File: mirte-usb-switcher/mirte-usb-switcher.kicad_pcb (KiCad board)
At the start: 2 copper layers, 18.4 x 27.4 mm, 5 parts, among them J1 Conn_02x02_Counter_Clockwise, U1 SIP32509DT-T1-GE3

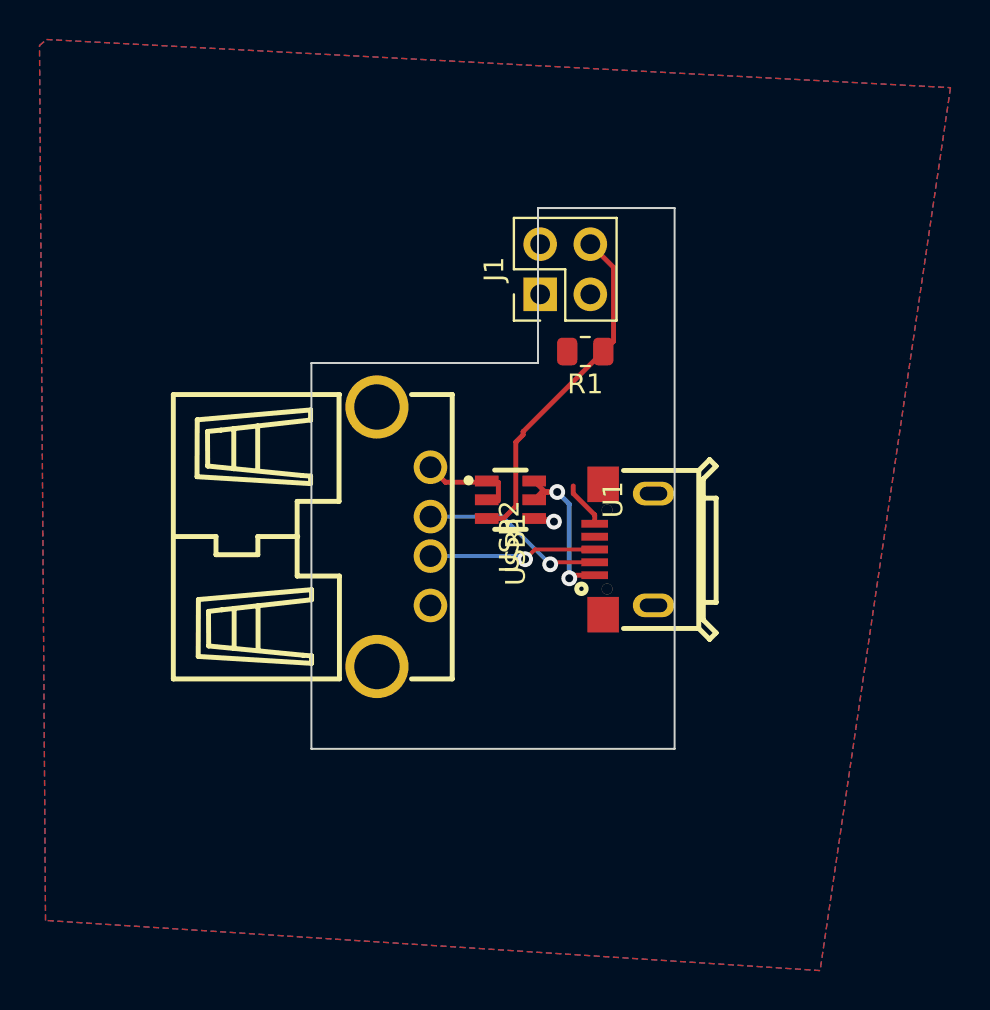
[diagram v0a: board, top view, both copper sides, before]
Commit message: move usb switcher
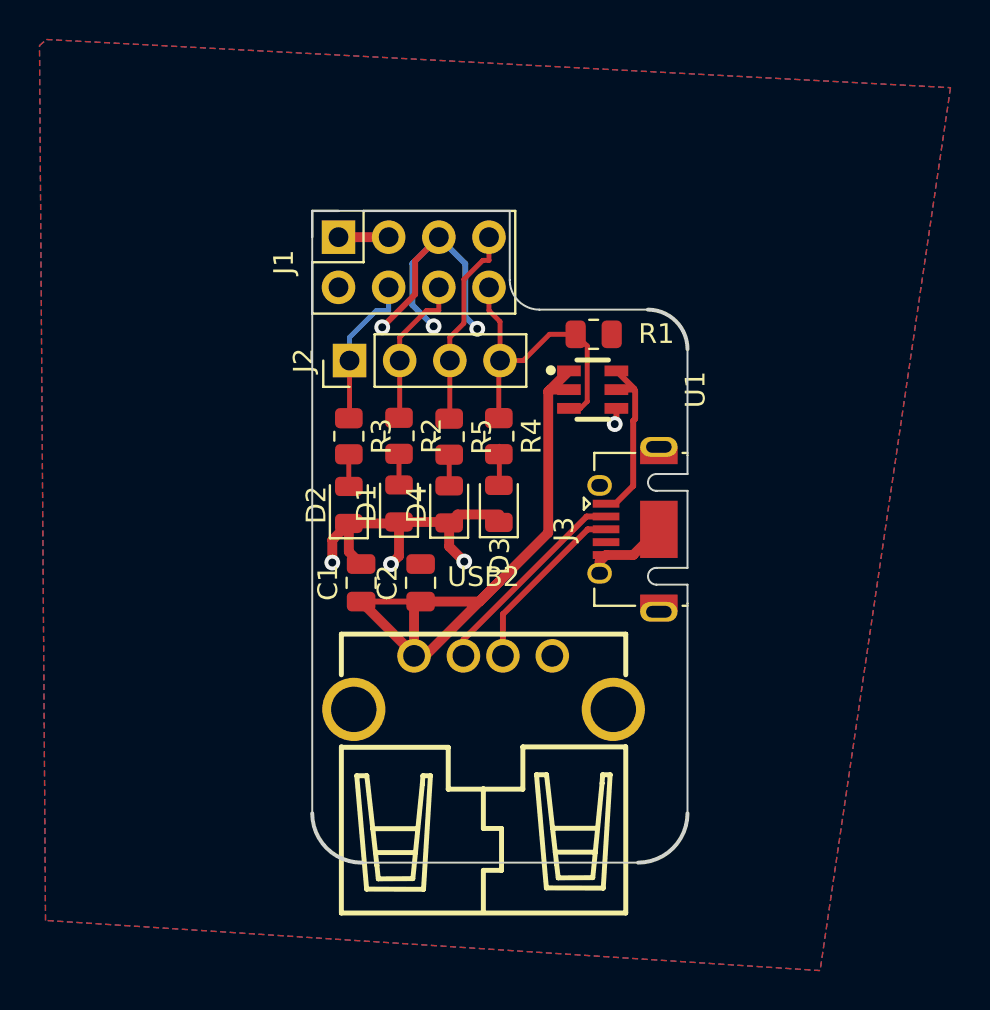
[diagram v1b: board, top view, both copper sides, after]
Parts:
- removed USB1: U254-051T-4BH83-S1S, lcsc:MICRO-USB-SMD_U254-051T-4BH83-S1S
- added C1: 10uF, Capacitor_SMD:C_0805_2012Metric, F.Cu at (55.0, 79.6)
- added C2: 100nF, Capacitor_SMD:C_0805_2012Metric, F.Cu at (58.1, 79.6)
- added D1: LED, LED_SMD:LED_0805_2012Metric, F.Cu at (57.0, 75.6)
- added D2: LED, LED_SMD:LED_0805_2012Metric, F.Cu at (54.4, 75.7)
- added D3: LED, LED_SMD:LED_0805_2012Metric, F.Cu at (62.0, 75.6)
- added D4: LED, LED_SMD:LED_0805_2012Metric, F.Cu at (59.5, 75.7)
- added J2: Conn_01x04_Pin, Connector_PinHeader_2.54mm:PinHeader_1x04_P2.54mm_Vertical, F.Cu at (54.5, 68.4)
- added J3: USB_B_Micro, Connector_USB:USB_Micro-AB_Molex_47590-0001, F.Cu at (70.1, 76.9)
- added R2: R, Resistor_SMD:R_0805_2012Metric, F.Cu at (57.0, 72.2)
- added R3: R, Resistor_SMD:R_0805_2012Metric, F.Cu at (54.4, 72.2)
- added R4: R, Resistor_SMD:R_0805_2012Metric, F.Cu at (62.0, 72.2)
- added R5: R, Resistor_SMD:R_0805_2012Metric, F.Cu at (59.5, 72.2)
- J1: value Conn_02x02_Counter_Clockwise -> Conn_02x04_Odd_Even; footprint Connector_PinHeader_2.54mm:PinHeader_2x02_P2.54mm_Vertical -> Connector_PinSocket_2.54mm:PinSocket_2x04_P2.54mm_Vertical
- moved J1 10.6 mm to (53.9, 62.1)
- moved USB2 8.43 mm to (61.2, 84.7), turned to 0 degrees
- moved U1 6.96 mm to (66.8, 69.8)
- moved R1 0.97 mm to (66.8, 67.0), turned to 0 degrees
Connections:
- net Net-(USB1-VBUS) renamed /VIN
- net Net-(USB2-VCC) renamed /VOUT
- J1 pad 1: unconnected-(J1-Pin_1-Pad1) -> +5V
- J1 pad 2: unconnected-(J1-Pin_2-Pad2) -> +3V3
- J1 pad 3: GND -> +5V
- J1 pad 4: /SW -> /GPIO4_B4
- R1 pad 1: /SW -> /GPIO4_A4
- U1 pad 3: /SW -> /GPIO4_A4
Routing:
- net GND: track 2.82 -> 39.0 mm, vias 1 -> 7
- net /VOUT: track 4.70 -> 33.3 mm
- net /SW: track 17.5 -> 0.00 mm
- net /GPIO4_A4: track 0.00 -> 16.0 mm
- net /GPIO0_D1: track 0.00 -> 10.2 mm
- net /GPIO4_B4: track 0.00 -> 7.83 mm
- net /GPIO4_B5: track 0.00 -> 7.81 mm
- net +5V: track 0.00 -> 2.54 mm
- net Net-(D2-A): track 0.00 -> 1.63 mm
- net Net-(D3-A): track 0.00 -> 1.58 mm
- net Net-(D4-A): track 0.00 -> 1.58 mm
- net Net-(D1-A): track 0.00 -> 1.57 mm
- net /D-: track 9.36 -> 10.6 mm, vias 1 -> 0
- net /D+: track 8.58 -> 9.11 mm, vias 1 -> 0
- net /VIN: track 8.70 -> 8.91 mm, vias 2 -> 0
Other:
- board size 18.4 x 27.4 mm -> 19 x 33 mm
